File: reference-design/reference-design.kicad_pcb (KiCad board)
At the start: 2 copper layers, 104 x 83.9 mm, 31 parts

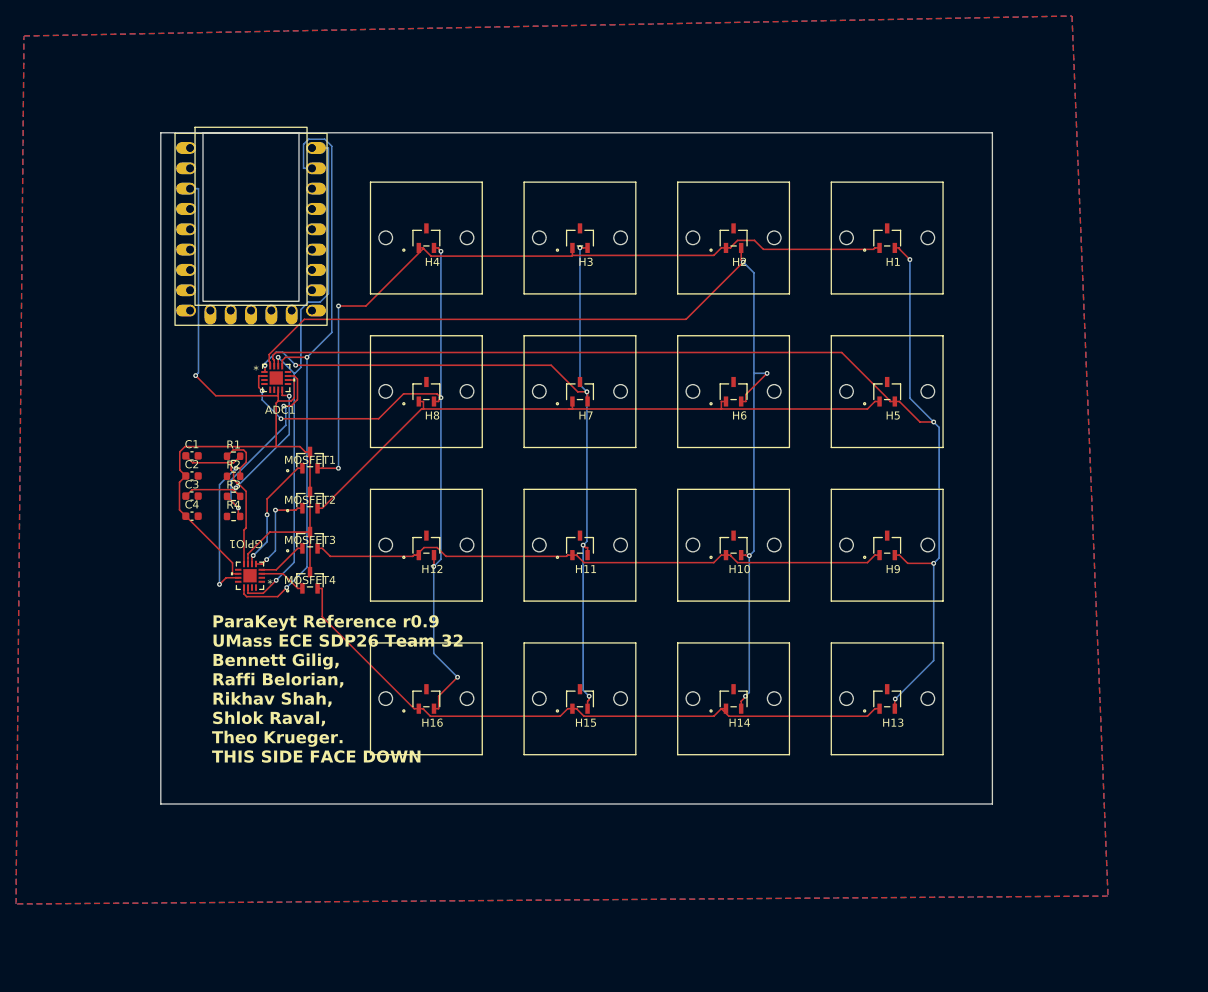
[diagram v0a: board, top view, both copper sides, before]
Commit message: stfupdate
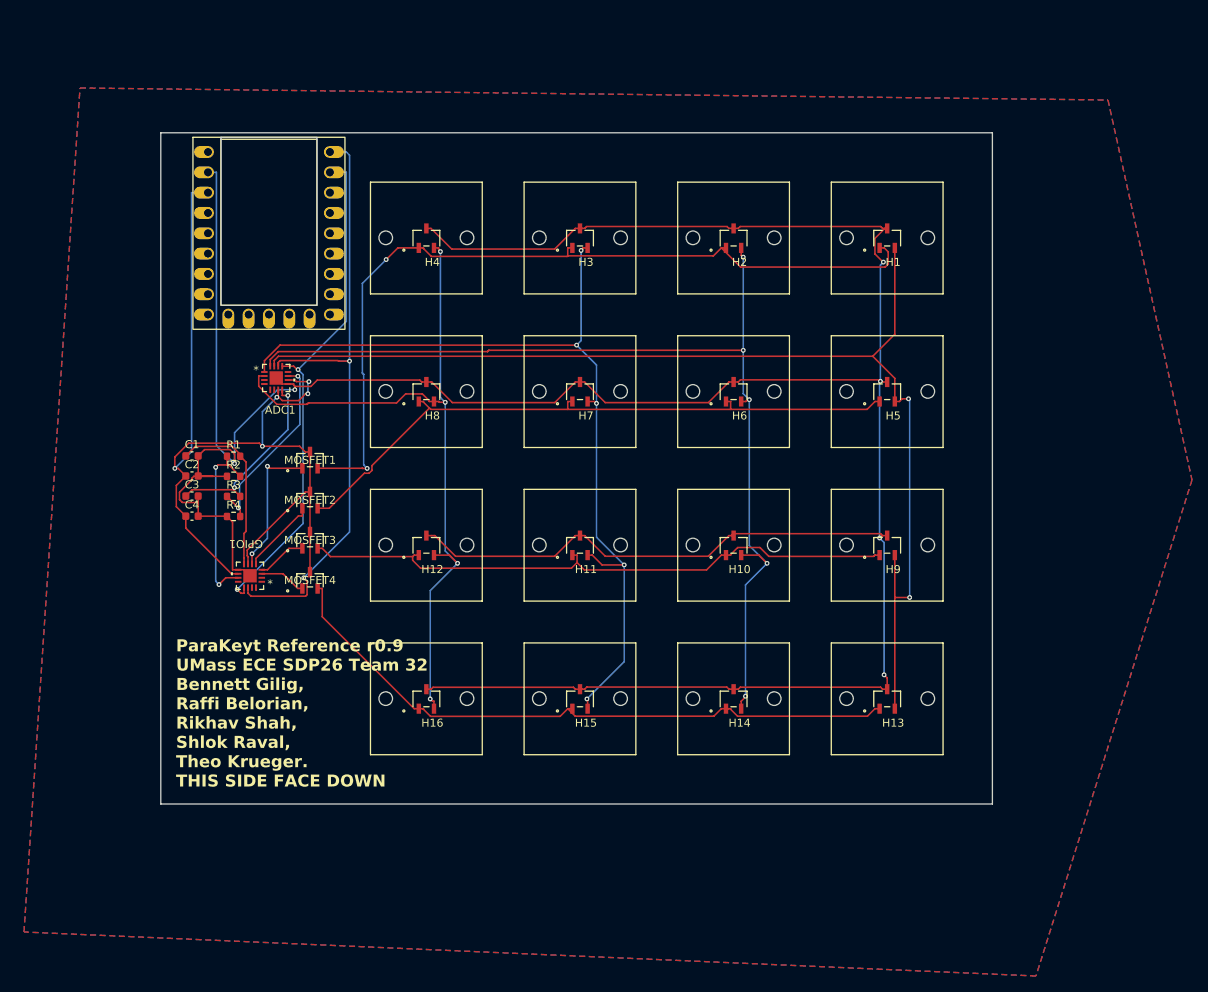
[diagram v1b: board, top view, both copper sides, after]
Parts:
- moved MCU1 2.30 mm to (25.6, 24.7)
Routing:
- net GND: track 0.00 -> 412.4 mm, vias 0 -> 6
- net i2c0_sda: track 68.6 -> 80.7 mm
- net i2c0_scl: track 76.4 -> 64.5 mm
- net col0: track 155.7 -> 145.0 mm, vias 4 -> 2
- net +3.3V: track 109.6 -> 119.2 mm, vias 1 -> 5
- net Net-(H1-VCC): track 96.9 -> 104.8 mm
- net col1: track 132.4 -> 125.7 mm, vias 4 -> 5
- net col2: track 106.4 -> 110.5 mm, vias 6 -> 5
- net row0: track 14.9 -> 18.9 mm
- net Net-(H10-VCC): track 73.6 -> 76.3 mm
- net Net-(GPIO1-ADDR): track 24.7 -> 22.4 mm
- net row1: track 11.7 -> 9.67 mm, vias 2 -> 0
- net col3: track 92.8 -> 91.7 mm, vias 6 -> 4
- net Net-(ADC1-ADDR): track 25.2 -> 24.2 mm
- net Net-(H5-VCC): track 80.2 -> 81.1 mm
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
